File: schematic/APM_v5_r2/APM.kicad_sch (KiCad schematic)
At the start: 23 parts, among them J14 ASDR_FFC, J18 WAVE_FFC, J2 CAN, J4 LCD_display

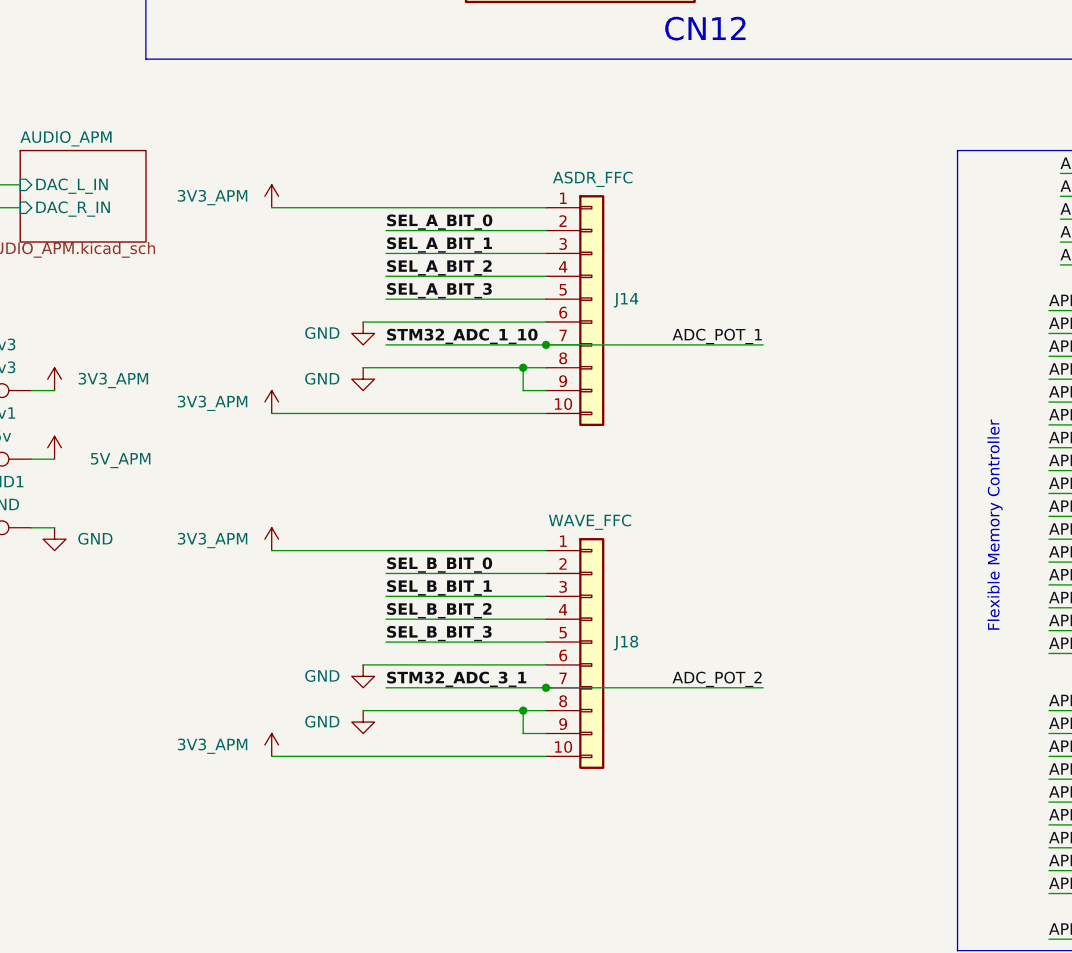
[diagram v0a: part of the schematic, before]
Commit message: trying APM placement
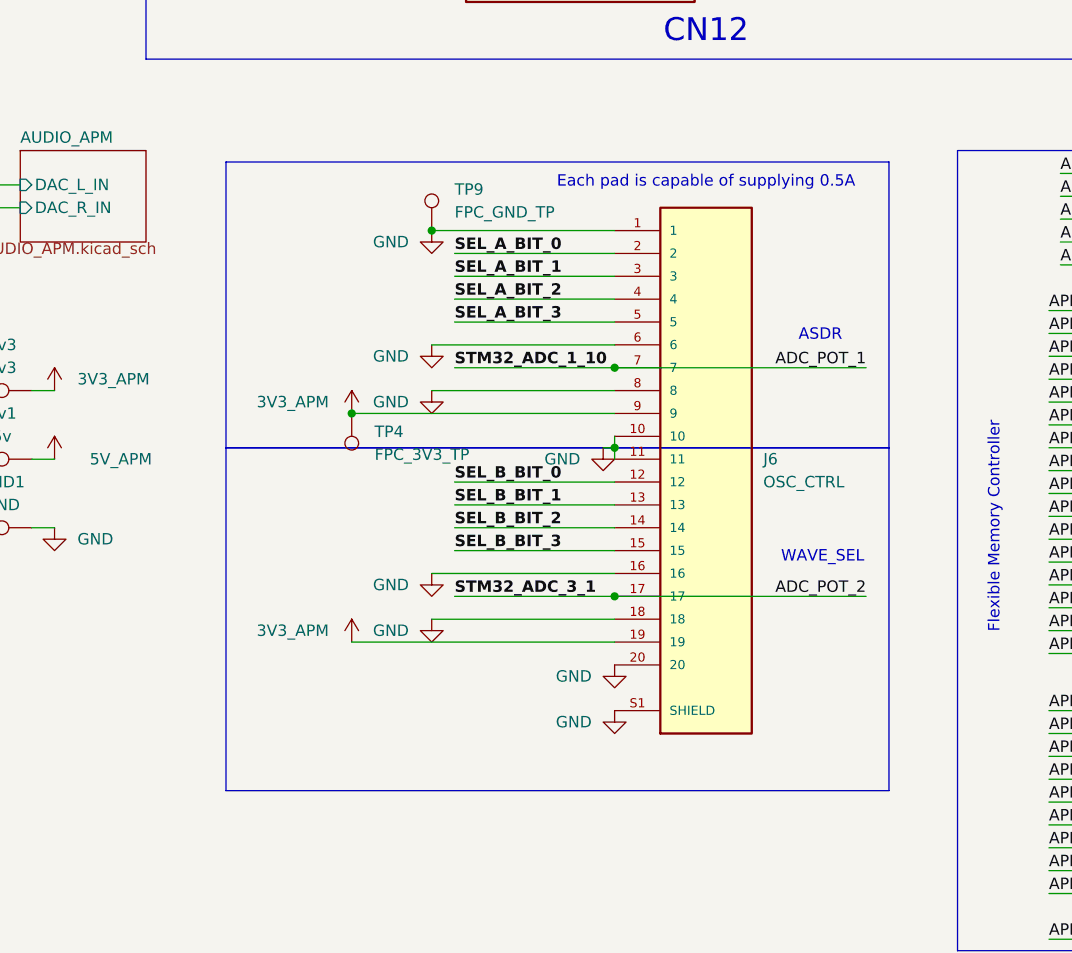
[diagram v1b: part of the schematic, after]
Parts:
- removed J14: ASDR_FFC, Connector_FFC-FPC:Hirose_FH12-10S-0.5SH_1x10-1MP_P0.50mm_Horizontal, symbol Connector_Generic:Conn_01x10
- removed J18: WAVE_FFC, Connector_FFC-FPC:Hirose_FH12-10S-0.5SH_1x10-1MP_P0.50mm_Horizontal, symbol Connector_Generic:Conn_01x10
- added J6: OSC_CTRL, my_footprints:GCT_FFC2B28-20-G, symbol FFC2B28-20-G:FFC2B28-20-G
- added TP4: FPC_3V3_TP, TestPoint:TestPoint_Pad_D1.0mm, symbol Connector:TestPoint
- added TP9: FPC_GND_TP, TestPoint:TestPoint_Pad_D1.0mm, symbol Connector:TestPoint
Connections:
- net 3V3_APM: now also J6.19, J6.9, TP4.1
- net ADC_POT_1: now also J6.7
- net ADC_POT_2: now also J6.17
- net GND: now also J6.1, J6.10, J6.11, J6.16, J6.18, J6.20, J6.6, J6.8, J6.S1 (SHIELD), J6.S2 (SHIELD), TP9.1
- net SEL_A_BIT_0: now also J6.2
- net SEL_A_BIT_1: now also J6.3
- net SEL_A_BIT_2: now also J6.4
- net SEL_A_BIT_3: now also J6.5
- net SEL_B_BIT_0: now also J6.12
- net SEL_B_BIT_1: now also J6.13
- net SEL_B_BIT_2: now also J6.14
- net SEL_B_BIT_3: now also J6.15
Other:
- note added: "ASDR"
- note added: "Each pad is capable of supplying 0.5A"
- note added: "WAVE_SEL"
